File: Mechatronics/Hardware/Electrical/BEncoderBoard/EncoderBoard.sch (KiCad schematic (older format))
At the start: 45 parts, among them IC1 RN4020-V_RM120, IC2 TP4056, IC3 DW01+G, J1 Conn_01x07_Male, J4 Barrel_Jack_Switch, J5 Batt+, J7 Batt-, Q1 FS8205, Q2 Q_PMOS_GSD, U1 STM32F103C8T6, U2 ITR1802A, U3 ITR1802B, U5 SSD1306OLED, U6 LTC2430, Y1 8Mhz

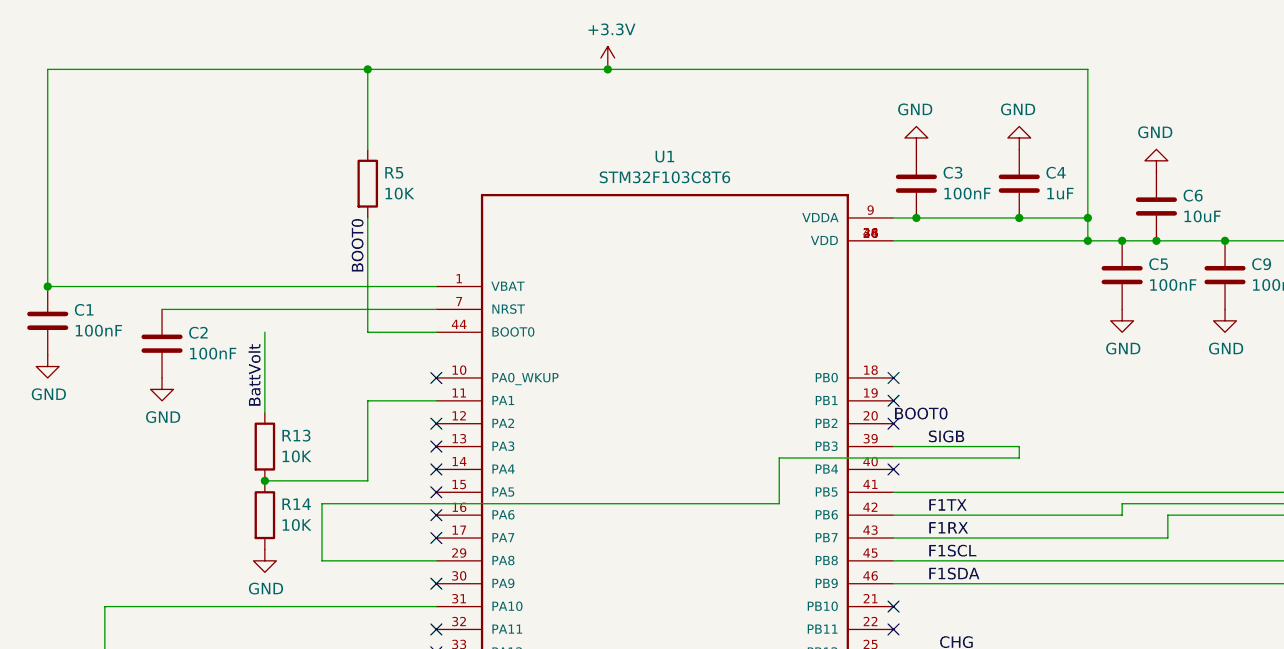
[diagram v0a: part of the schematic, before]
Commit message: Added changes
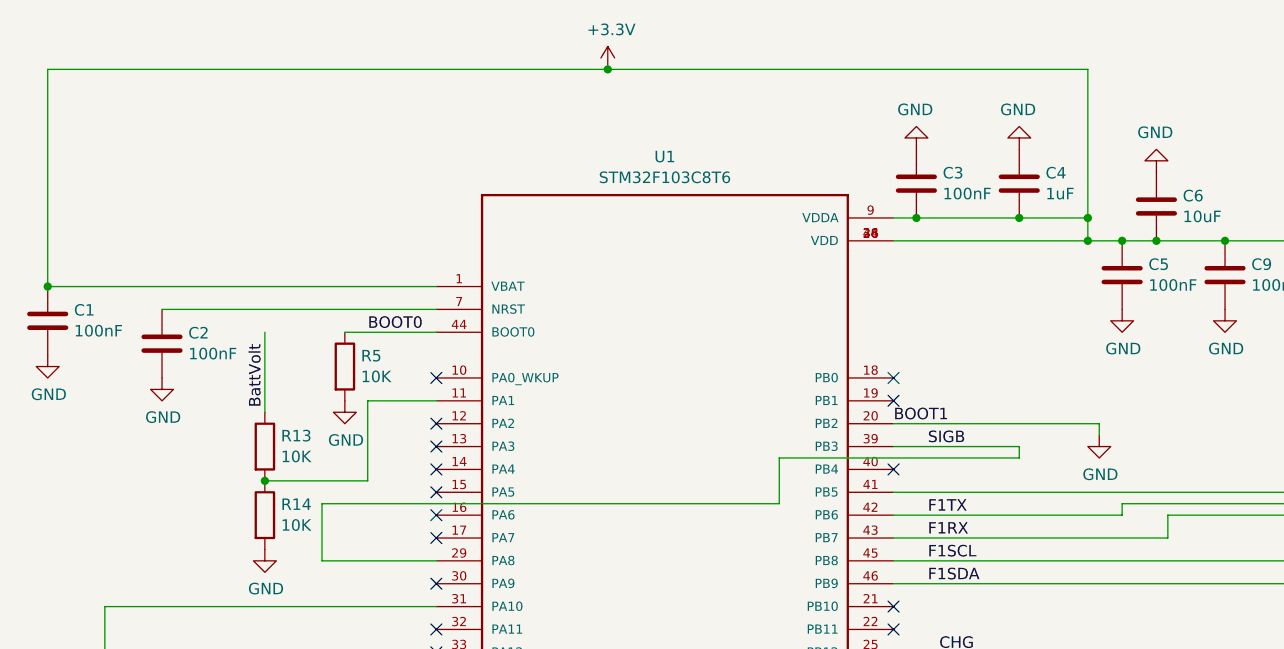
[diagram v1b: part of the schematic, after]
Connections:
- net labels added: BOOT1
- wire segments 167 -> 166
- no-connect marks 37 -> 36
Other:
- moved on the sheet: R5
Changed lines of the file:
@@
 L Device:R R5
 U 1 1 5D4A832E
-P 2150 1400
-F 0 "R5" H 2220 1446 50  0000 L CNN
-F 1 "10K" H 2220 1355 50  0000 L CNN
-F 2 "Encoder:R_0603_1608Metric_Pad1.05x0.95mm_HandSolder" V 2080 1400 50  0001 C CNN
-F 3 "~" H 2150 1400 50  0001 C CNN
-	1    2150 1400
-	1    0    0    -1
-$EndComp
-Wire Wire Line
-	2150 1250 2150 900
-Wire Wire Line
-	2150 1550 2150 2050
-Wire Wire Line
-	2150 2050 2450 2050
+P 2050 2200
+F 0 "R5" H 2120 2246 50  0000 L CNN
+F 1 "10K" H 2120 2155 50  0000 L CNN
+F 2 "Encoder:R_0603_1608Metric_Pad1.05x0.95mm_HandSolder" V 1980 2200 50  0001 C CNN
+F 3 "~" H 2050 2200 50  0001 C CNN
+	1    2050 2200
+	1    0    0    -1
+$EndComp
 Text Label 2100 3550 0    50   ~ 0
 SWDIO
@@
 	1    0    0    -1
 $EndComp
-Connection ~ 2150 900
-Wire Wire Line
-	2150 900  3200 900
 Wire Wire Line
 	4450 3050 6900 3050
@@
 NoConn ~ 4450 2250
 NoConn ~ 4450 2350
-NoConn ~ 4450 2450
 NoConn ~ 4450 2650
 Wire Wire Line
@@
 NoConn ~ 4450 3250
 NoConn ~ 4450 3350
-Text Label 2150 1550 3    50   ~ 0
+Text Label 2150 2050 0    50   ~ 0
 BOOT0
 Text Label 4450 2450 0    50   ~ 0
-BOOT0
-Wire Wire Line
-	750  900  2150 900
+BOOT1
 Text Label 1700 2100 3    50   ~ 0
 BattVolt
@@
 Wire Wire Line
 	1700 2400 1700 2050
+Wire Wire Line
+	4450 2450 5350 2450
+Wire Wire Line
+	5350 2450 5350 2500
+$Comp
+L power:GND #PWR0102
+U 1 1 5D535B59
+P 5350 2500
+F 0 "#PWR0102" H 5350 2250 50  0001 C CNN
+F 1 "GND" H 5355 2327 50  0000 C CNN
+F 2 "" H 5350 2500 50  0001 C CNN
+F 3 "" H 5350 2500 50  0001 C CNN
+	1    5350 2500
+	1    0    0    -1
+$EndComp
+Wire Wire Line
+	750  900  3200 900
+Wire Wire Line
+	2050 2050 2450 2050
+$Comp
+L power:GND #PWR?
+U 1 1 5D5484B5
+P 2050 2350
+F 0 "#PWR?" H 2050 2100 50  0001 C CNN
+F 1 "GND" H 2055 2177 50  0000 C CNN
+F 2 "" H 2050 2350 50  0001 C CNN
+F 3 "" H 2050 2350 50  0001 C CNN
+	1    2050 2350
+	1    0    0    -1
+$EndComp
 $EndSCHEMATC
